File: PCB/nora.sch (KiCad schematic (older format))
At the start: 215 parts, among them J1 USB_C_Receptacle_USB2.0, J3 Conn_01x02, J5 Conn_02x03_Odd_Even, U1 ATmega32U4-MU, U2 24LC64, U3 ATmega32U4-AU-Dummy, Y1 16MHz

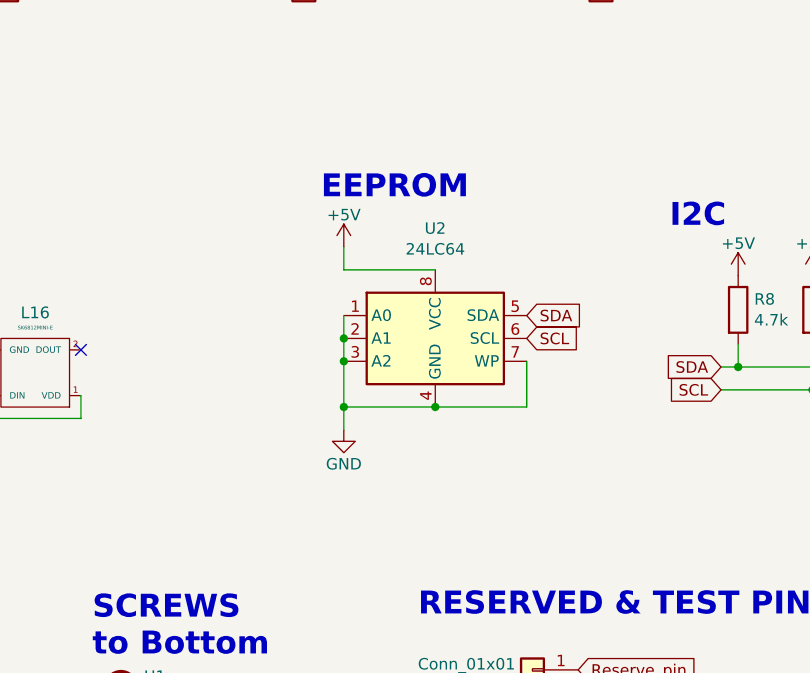
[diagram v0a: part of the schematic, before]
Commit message: ロゴ追加
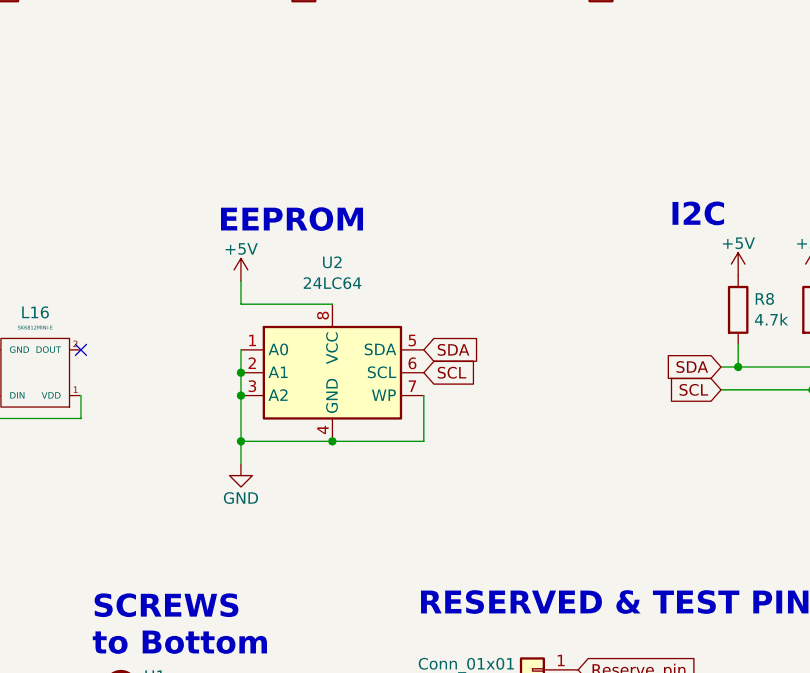
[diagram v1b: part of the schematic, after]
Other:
- moved on the sheet: U2
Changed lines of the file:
@@
 	-1   0    0    1
 $EndComp
-Text GLabel 9750 8625 2    50   Input ~ 0
+Text GLabel 9300 8775 2    50   Input ~ 0
 SDA
-Text GLabel 9750 8725 2    50   Input ~ 0
+Text GLabel 9300 8875 2    50   Input ~ 0
 SCL
-Connection ~ 8950 9025
+Connection ~ 8500 9175
 Wire Wire Line
-	8950 9025 8950 9125
+	8500 9175 8500 9275
 Wire Wire Line
-	8950 8425 9350 8425
+	8500 8575 8900 8575
 Wire Wire Line
-	8950 8325 8950 8425
+	8500 8475 8500 8575
 $Comp
 L power:+5V #PWR0102
 U 1 1 60AF154D
-P 8950 8325
-F 0 "#PWR0102" H 8950 8175 50  0001 C CNN
-F 1 "+5V" H 8950 8465 50  0000 C CNN
-F 2 "" H 8950 8325 50  0001 C CNN
-F 3 "" H 8950 8325 50  0001 C CNN
-	1    8950 8325
+P 8500 8475
+F 0 "#PWR0102" H 8500 8325 50  0001 C CNN
+F 1 "+5V" H 8500 8615 50  0000 C CNN
+F 2 "" H 8500 8475 50  0001 C CNN
+F 3 "" H 8500 8475 50  0001 C CNN
+	1    8500 8475
 	1    0    0    -1
 $EndComp
 Wire Wire Line
-	9750 9025 9350 9025
+	9300 9175 8900 9175
 Wire Wire Line
-	9750 8825 9750 9025
-Connection ~ 9350 9025
+	9300 8975 9300 9175
+Connection ~ 8900 9175
 Wire Wire Line
-	8950 8825 8950 9025
-Connection ~ 8950 8825
+	8500 8975 8500 9175
+Connection ~ 8500 8975
 Wire Wire Line
-	8950 8725 8950 8825
-Connection ~ 8950 8725
+	8500 8875 8500 8975
+Connection ~ 8500 8875
 Wire Wire Line
-	8950 9025 9350 9025
+	8500 9175 8900 9175
 Wire Wire Line
-	8950 8625 8950 8725
+	8500 8775 8500 8875
 $Comp
 L power:GND #PWR0101
 U 1 1 60B24F18
-P 8950 9125
-F 0 "#PWR0101" H 8950 8875 50  0001 C CNN
-F 1 "GND" H 8950 8975 50  0000 C CNN
-F 2 "" H 8950 9125 50  0001 C CNN
-F 3 "" H 8950 9125 50  0001 C CNN
-	1    8950 9125
+P 8500 9275
+F 0 "#PWR0101" H 8500 9025 50  0001 C CNN
+F 1 "GND" H 8500 9125 50  0000 C CNN
+F 2 "" H 8500 9275 50  0001 C CNN
+F 3 "" H 8500 9275 50  0001 C CNN
+	1    8500 9275
 	1    0    0    -1
 $EndComp
@@
 L Memory_EEPROM:24LC64 U2
 U 1 1 60AF01F9
-P 9350 8725
-F 0 "U2" H 9350 9206 50  0000 C CNN
-F 1 "24LC64" H 9350 9115 50  0000 C CNN
-F 2 "Package_SO:SO-8_3.9x4.9mm_P1.27mm" H 9350 8725 50  0001 C CNN
-F 3 "http://ww1.microchip.com/downloads/en/DeviceDoc/21189f.pdf" H 9350 8725 50  0001 C CNN
-F 4 "C79988" H 9350 8725 50  0001 C CNN "LCSC"
-	1    9350 8725
+P 8900 8875
+F 0 "U2" H 8900 9356 50  0000 C CNN
+F 1 "24LC64" H 8900 9265 50  0000 C CNN
+F 2 "Package_SO:SO-8_3.9x4.9mm_P1.27mm" H 8900 8875 50  0001 C CNN
+F 3 "http://ww1.microchip.com/downloads/en/DeviceDoc/21189f.pdf" H 8900 8875 50  0001 C CNN
+F 4 "C79988" H 8900 8875 50  0001 C CNN "LCSC"
+	1    8900 8875
 	1    0    0    -1
 $EndComp
@@
 Text Notes 12425 7825 0    100  ~ 20
 USB
-Text Notes 8850 8125 0    100  ~ 20
+Text Notes 8400 8275 0    100  ~ 20
 EEPROM
 Text Notes 10375 8250 0    100  ~ 20
@@
 Text GLabel 18075 3175 2    50   Input ~ 0
 SDA
-Text GLabel 18075 2775 2    50   Input ~ 0
-Reserve_pin
 Text GLabel 18075 3375 2    50   Input ~ 0
 col1
@@
 Text GLabel 15325 3275 2    50   Input ~ 0
 row2
+Text GLabel 18075 2775 2    50   Input ~ 0
+Reserve_pin
 $EndSCHEMATC
